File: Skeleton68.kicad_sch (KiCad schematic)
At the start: 224 parts, among them J1 USB_C_Receptacle_USB2.0, SW1 SW_PUSH, SW10 SW_PUSH, SW11 SW_PUSH, SW12 SW_PUSH, SW13 SW_PUSH, SW14 SW_PUSH, SW15 SW_PUSH, SW16 SW_PUSH, SW17 SW_PUSH, SW18 SW_PUSH, SW19 SW_PUSH, SW2 SW_PUSH, SW20 SW_PUSH, SW21 SW_PUSH, SW22 SW_PUSH, SW23 SW_PUSH, SW24 SW_PUSH, SW25 SW_PUSH, SW26 SW_PUSH, SW27 SW_PUSH, SW28 SW_PUSH, SW29 SW_PUSH, SW3 SW_PUSH, SW30 SW_PUSH, SW31 SW_PUSH, SW32 SW_PUSH, SW33 SW_PUSH, SW34 SW_PUSH, SW35 SW_PUSH, SW36 SW_PUSH, SW37 SW_PUSH, SW38 SW_PUSH, SW39 SW_PUSH, SW4 SW_PUSH, SW40 SW_PUSH, SW41 SW_PUSH, SW42 SW_PUSH, SW43 SW_PUSH, SW44 SW_PUSH, SW45 SW_PUSH, SW46 SW_PUSH, SW47 SW_PUSH, SW48 SW_PUSH, SW49 SW_PUSH, SW5 SW_PUSH, SW50 SW_PUSH, SW51 SW_PUSH, SW52 SW_PUSH, SW53 SW_PUSH, SW54 SW_PUSH, SW55 SW_PUSH, SW56 SW_PUSH, SW57 SW_PUSH, SW58 SW_PUSH, SW59 SW_PUSH, SW6 SW_PUSH, SW60 SW_PUSH, SW61 SW_PUSH, SW62 SW_PUSH, SW63 SW_PUSH, SW64 SW_PUSH, SW65 SW_PUSH, SW66 SW_PUSH, SW67 SW_PUSH, SW68 SW_PUSH, SW7 SW_PUSH, SW8 SW_PUSH, SW9 SW_PUSH, U1 ATmega32U4-M, U2 PRTR5V0U2X, Y1 Crystal_GND24

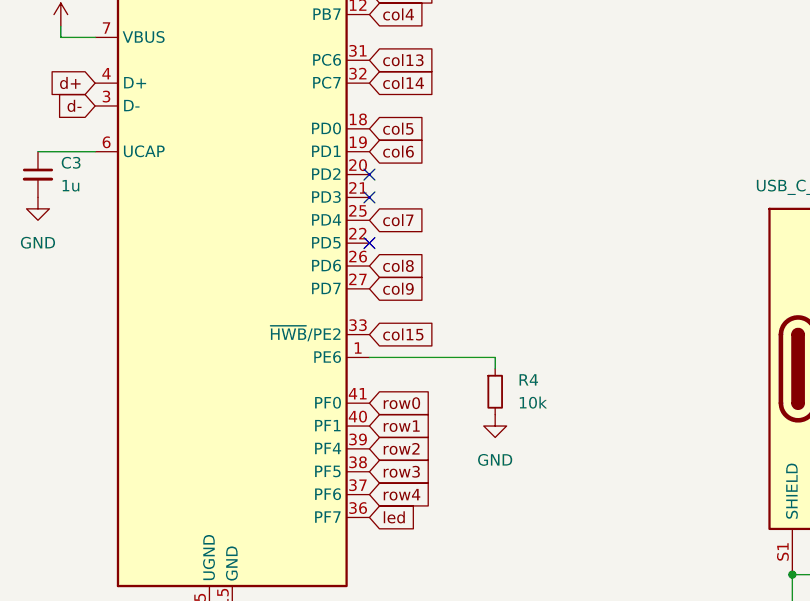
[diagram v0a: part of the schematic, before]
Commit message: trial
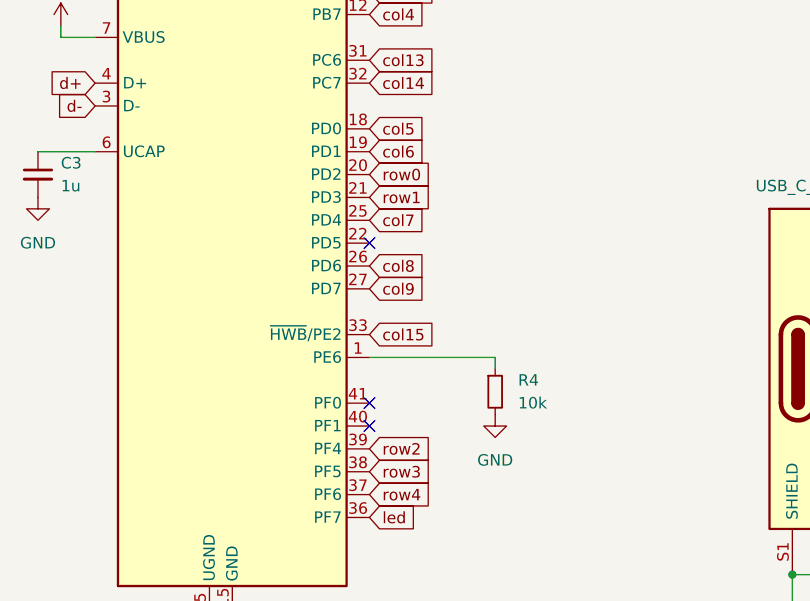
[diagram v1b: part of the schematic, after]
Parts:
- SW1, SW10, SW11, SW12, SW13, SW15, SW17, SW18, SW19, SW2, SW20, SW21, SW22, SW23, SW24, SW25, SW26, SW27, SW28, SW3, SW30, SW32, SW33, SW34, SW35, SW36, SW37, SW38, SW39, SW4, SW40, SW41, SW42, SW44, SW46, SW47, SW48, SW49, SW5, SW50, SW51, SW52, SW53, SW54, SW55, SW56, SW58, SW6, SW62, SW66, SW67, SW68, SW7, SW8, SW9: footprint MX_Only:MXOnly-1U-Hotswap -> Custom:MXOnly-1U-Hotswap
- SW14: footprint MX_Only:MXOnly-2U-Hotswap -> Custom:MXOnly-2U-Hotswap
- SW16, SW29, SW59, SW60, SW64, SW65: footprint MX_Only:MXOnly-1.5U-Hotswap -> Custom:MXOnly-1.5U-Hotswap
- SW31, SW57: footprint MX_Only:MXOnly-1.75U-Hotswap -> Custom:MXOnly-1.75U-Hotswap
- SW43, SW45: footprint MX_Only:MXOnly-2.25U-Hotswap -> Custom:MXOnly-2.25U-Hotswap
- SW61: footprint MX_Only:MXOnly-2U-Hotswap-ReversedStabilizers -> Custom:MXOnly-2U-Hotswap-ReversedStabilizers
- SW63: footprint MX_Only:MXOnly-2.75U-Hotswap-ReversedStabilizers -> Custom:MXOnly-2.75U-Hotswap-ReversedStabilizers
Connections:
- net row0: now also U1.20 (PD2); no longer U1.41 (PF0)
- net row1: now also U1.21 (PD3); no longer U1.40 (PF1)
